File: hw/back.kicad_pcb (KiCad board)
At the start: 2 copper layers, 110 x 55 mm, 77 parts, among them J1 IDC_02X13, J2 FC681495, J3 N42GK-04, Q1 BSC080N03MS, U1 OSRB38C9BA, U2 MCP1826S, U3 MCP1826S, U4 BQ24192, U5 LTC1871, U6 LTC2941CMS8E

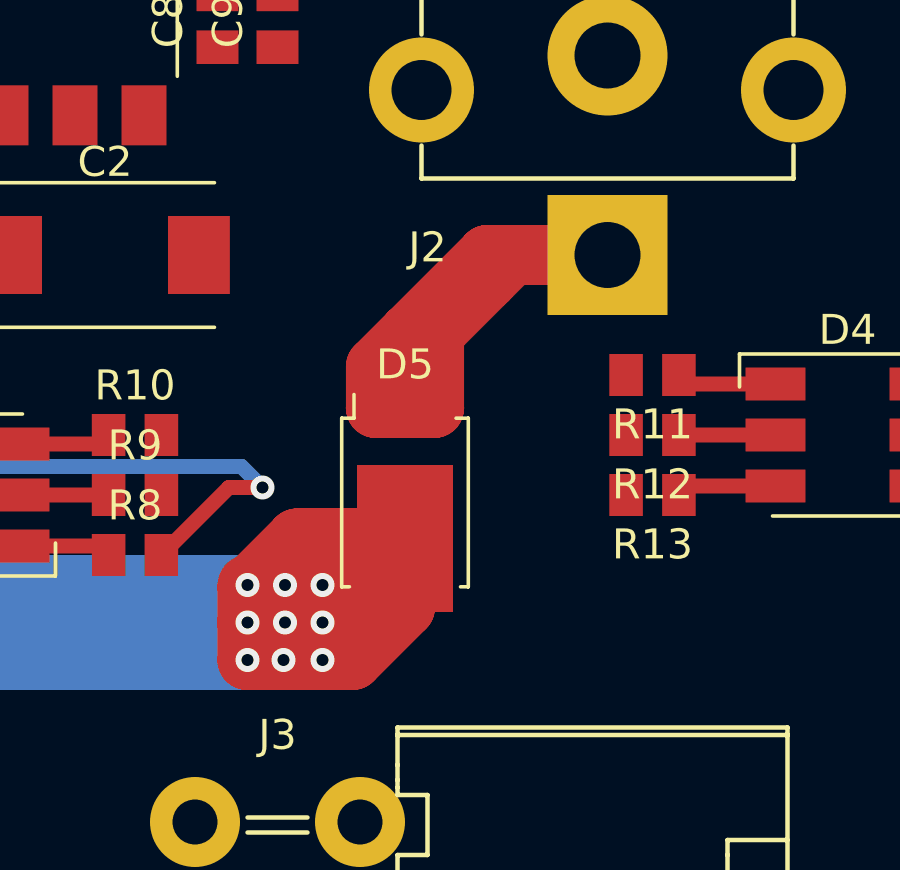
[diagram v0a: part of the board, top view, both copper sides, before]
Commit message: updated pcb
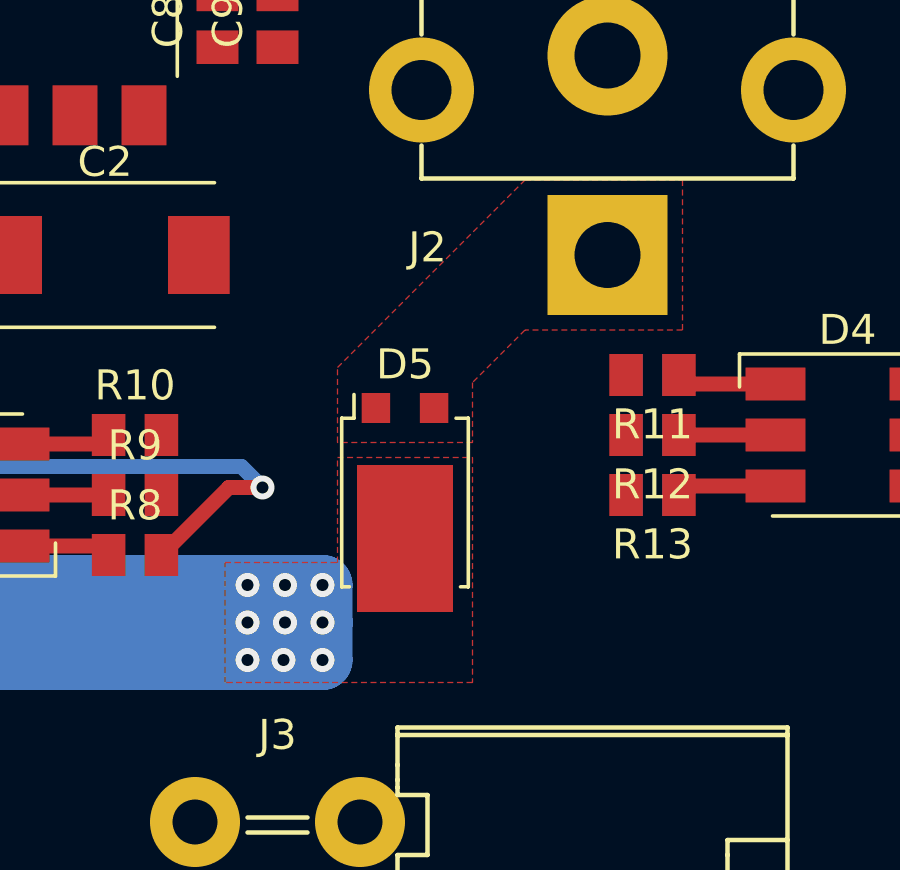
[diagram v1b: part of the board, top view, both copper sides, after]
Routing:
- net /charger/ADAPTER: track 191.2 -> 146.6 mm
- net Net-(D5-Pad1): track 25.3 -> 0.00 mm
- added copper zone on F.Cu, net /charger/ADAPTER
- added copper zone on F.Cu, net Net-(D5-Pad1)
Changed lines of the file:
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@@
     (thickness 1.6)
     (drawings 6)
-    (tracks 478)
+    (tracks 443)
     (zones 0)
     (modules 77)
@@
     (mod_text_size 1 1)
     (mod_text_width 0.15)
-    (pad_size 0.85 0.3)
-    (pad_drill 0)
+    (pad_size 4 4)
+    (pad_drill 2.2)
     (pad_to_mask_clearance 0.2)
     (aux_axis_origin 0 0)
@@
       (net 5 GND))
     (pad 1 thru_hole rect (at 0 -10.25 180) (size 4 4) (drill 2.2) (layers *.Cu *.Mask)
-      (net 8 "Net-(D5-Pad1)"))
+      (net 8 "Net-(D5-Pad1)") (zone_connect 2))
     (pad 2 thru_hole circle (at 0 -3.6 180) (size 4 4) (drill 2.2) (layers *.Cu *.Mask)
       (net 5 GND))
@@
       (net 8 "Net-(D5-Pad1)"))
     (pad 3 smd rect (at 0 1.2) (size 3.2 4.9) (layers F.Cu F.Mask)
-      (net 24 /charger/ADAPTER))
+      (net 24 /charger/ADAPTER) (zone_connect 2))
     (pad 1 smd rect (at -0.97 -3.15) (size 0.95 1) (layers F.Cu F.Paste F.Mask)
       (net 8 "Net-(D5-Pad1)"))
@@
   (segment (start 171.2 112.5) (end 172.5 112.5) (width 2) (layer B.Cu) (net 24))
   (segment (start 170 112.5) (end 171.2 112.5) (width 2) (layer B.Cu) (net 24))
-  (segment (start 171.2 112.5) (end 172.5 112.5) (width 2) (layer F.Cu) (net 24))
-  (segment (start 171.25 111.25) (end 171.25 110) (width 2) (layer F.Cu) (net 24))
-  (segment (start 172.5 111.25) (end 171.25 111.25) (width 2) (layer F.Cu) (net 24))
-  (segment (start 171.25 110) (end 172.5 110) (width 2) (layer F.Cu) (net 24))
-  (segment (start 170 110) (end 171.25 110) (width 2) (layer F.Cu) (net 24))
   (via (at 172.5 110) (size 0.8) (drill 0.4) (layers F.Cu B.Cu) (net 24))
   (via (at 171.25 110) (size 0.8) (drill 0.4) (layers F.Cu B.Cu) (net 24))
@@
   (via (at 172.5 111.25) (size 0.8) (drill 0.4) (layers F.Cu B.Cu) (net 24))
   (via (at 171.25 111.25) (size 0.8) (drill 0.4) (layers F.Cu B.Cu) (net 24))
-  (segment (start 170 111.25) (end 170 111.3) (width 2) (layer F.Cu) (net 24))
-  (segment (start 170 111.3) (end 171.2 112.5) (width 2) (layer F.Cu) (net 24))
   (via (at 171.2 112.5) (size 0.8) (drill 0.4) (layers F.Cu B.Cu) (net 24))
   (via (at 170 111.25) (size 0.8) (drill 0.4) (layers F.Cu B.Cu) (net 24))
-  (segment (start 171.65 108.45) (end 175.25 108.45) (width 2) (layer F.Cu) (net 24))
-  (segment (start 175.25 110.75) (end 173.5 112.5) (width 2) (layer F.Cu) (net 24))
-  (segment (start 173.5 112.5) (end 171.2 112.5) (width 2) (layer F.Cu) (net 24))
-  (segment (start 175.25 108.45) (end 175.25 110.75) (width 2) (layer F.Cu) (net 24))
-  (segment (start 172.75 108.45) (end 175.25 108.45) (width 2) (layer F.Cu) (net 24))
-  (segment (start 170 112.5) (end 170 111.25) (width 2) (layer F.Cu) (net 24))
-  (segment (start 170 111.2) (end 172.75 108.45) (width 2) (layer F.Cu) (net 24))
-  (segment (start 171.65 108.45) (end 172.75 108.45) (width 2) (layer F.Cu) (net 24))
-  (segment (start 170 111.25) (end 170 110.1) (width 2) (layer F.Cu) (net 24))
-  (segment (start 170 111.25) (end 170 111.2) (width 2) (layer F.Cu) (net 24))
-  (segment (start 170 110.1) (end 171.65 108.45) (width 2) (layer F.Cu) (net 24))
-  (segment (start 170 112.5) (end 171.2 112.5) (width 2) (layer F.Cu) (net 24))
-  (segment (start 171.2 112.5) (end 175.25 108.45) (width 2) (layer F.Cu) (net 24))
-  (segment (start 175.25 109.25) (end 172 112.5) (width 2) (layer F.Cu) (net 24))
-  (segment (start 172 112.5) (end 170 112.5) (width 2) (layer F.Cu) (net 24))
   (via (at 170 112.5) (size 0.8) (drill 0.4) (layers F.Cu B.Cu) (net 24))
   (segment (start 175.25 108.45) (end 175.25 109.25) (width 2) (layer F.Cu) (net 24))
@@
   (segment (start 155.25 94.3) (end 155.2 94.35) (width 1) (layer F.Cu) (net 4))
   (segment (start 161.943309 94.35) (end 161.95 94.343309) (width 1) (layer F.Cu) (net 4))
-  (segment (start 182 99) (end 178.82 99) (width 2) (layer F.Cu) (net 8))
-  (segment (start 178.82 99) (end 178 99.82) (width 2) (layer F.Cu) (net 8))
-  (segment (start 174.28 104.1) (end 174.28 102.72) (width 2) (layer F.Cu) (net 8))
-  (segment (start 174.28 102.72) (end 175.4 101.6) (width 2) (layer F.Cu) (net 8))
-  (segment (start 176.22 104.1) (end 176.22 101.6) (width 2) (layer F.Cu) (net 8))
-  (segment (start 176.22 101.6) (end 178 99.82) (width 2) (layer F.Cu) (net 8))
-  (segment (start 178 99.82) (end 178 99) (width 2) (layer F.Cu) (net 8))
-  (segment (start 174.28 104.1) (end 175.2 104.1) (width 2) (layer F.Cu) (net 8))
-  (segment (start 175.2 104.1) (end 176.22 104.1) (width 2) (layer F.Cu) (net 8))
-  (segment (start 175.4 101.6) (end 175.4 103.9) (width 2) (layer F.Cu) (net 8))
-  (segment (start 175.4 103.9) (end 175.2 104.1) (width 2) (layer F.Cu) (net 8))
-  (segment (start 182 99) (end 178 99) (width 2) (layer F.Cu) (net 8))
-  (segment (start 178 99) (end 175.4 101.6) (width 2) (layer F.Cu) (net 8))
   (segment (start 187.6 103.3) (end 184.68 103.3) (width 0.5) (layer F.Cu) (net 9))
   (segment (start 184.68 103.3) (end 184.38 103) (width 0.5) (layer F.Cu) (net 9))
@@
       )
     )
+  )
+  (zone (net 24) (net_name /charger/ADAPTER) (layer F.Cu) (hatch edge 0.508)
+    (priority 1)
+    (connect_pads (clearance 0.508))
+    (min_thickness 0.254)
+    (fill yes (arc_segments 16) (thermal_gap 0.508) (thermal_bridge_width 0.508))
+    (polygon
+      (pts
+        (xy 169.25 109.25) (xy 173 109.25) (xy 173 105.75) (xy 177.5 105.75) (xy 177.5 113.25)
+        (xy 169.25 113.25)
+      )
+    )
+  )
+  (zone (net 8) (net_name "Net-(D5-Pad1)") (layer F.Cu) (hatch edge 0.508)
+    (priority 2)
+    (connect_pads (clearance 0.508))
+    (min_thickness 0.254)
+    (fill yes (arc_segments 16) (thermal_gap 0.508) (thermal_bridge_width 0.508))
+    (polygon
+      (pts
+        (xy 173 102.75) (xy 179.25 96.5) (xy 184.5 96.5) (xy 184.5 101.5) (xy 179.25 101.5)
+        (xy 177.5 103.25) (xy 177.5 105.25) (xy 173 105.25)
+      )
+    )

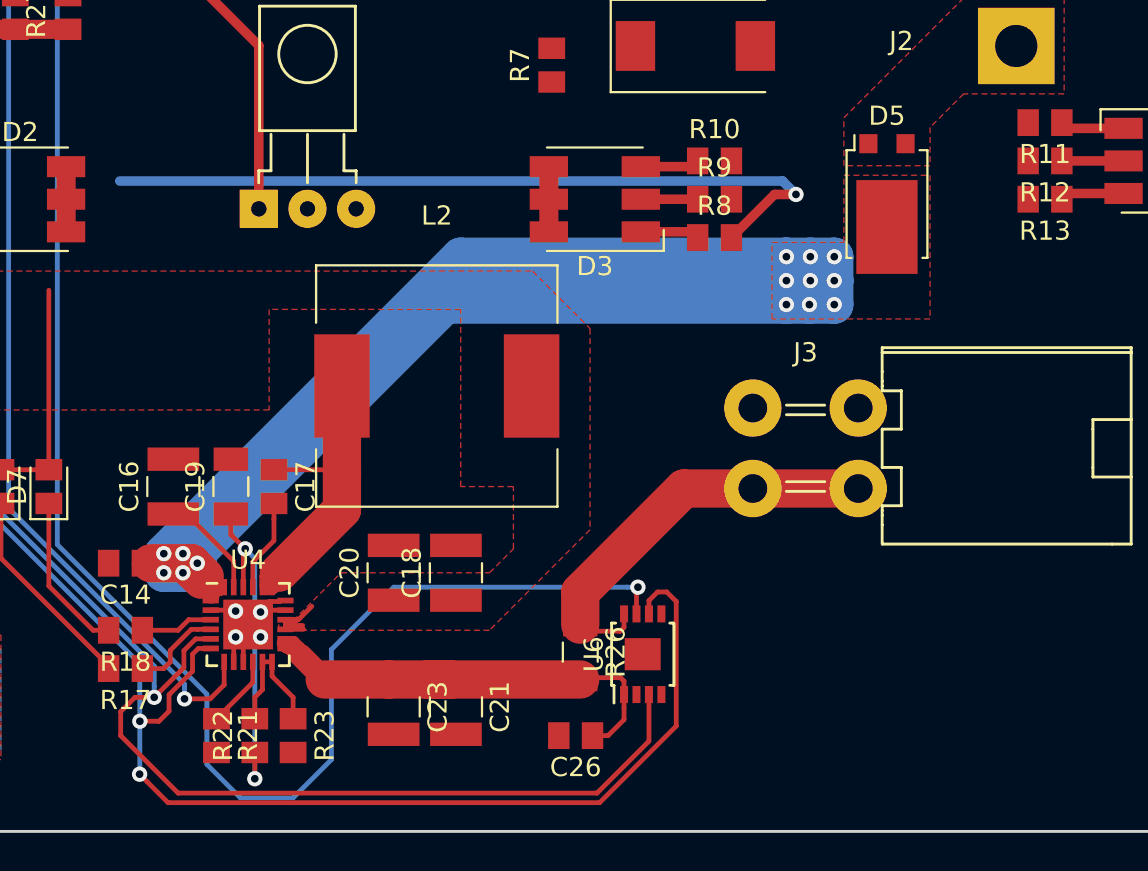
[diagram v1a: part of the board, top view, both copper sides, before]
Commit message: updated pcb
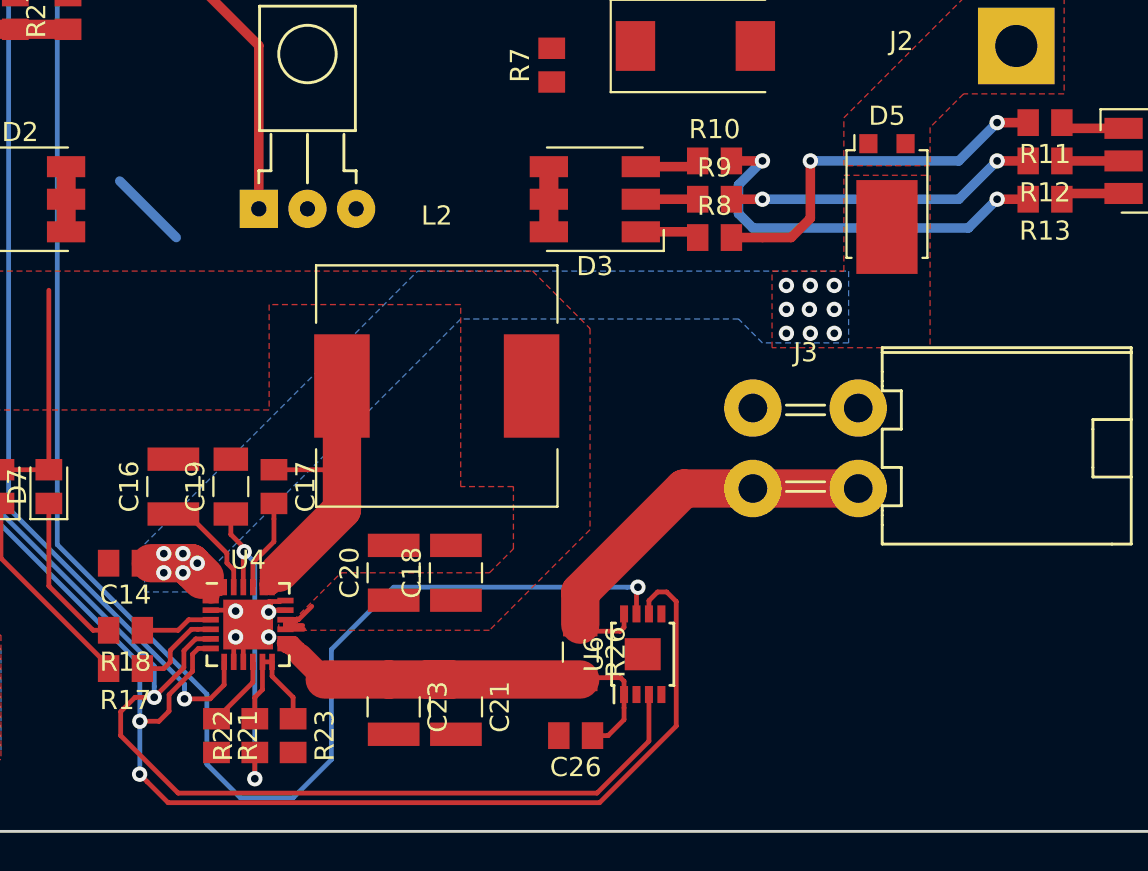
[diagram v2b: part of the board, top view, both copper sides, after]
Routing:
- net /charger/ADAPTER: track 146.6 -> 15.4 mm
- net /PWM_R: track 32.0 -> 52.9 mm, vias 0 -> 2
- net /PWM_G: track 42.5 -> 58.8 mm, vias 1 -> 3
- net /PWM_B: track 86.4 -> 70.4 mm, vias 2 -> 3
- added copper zone on B.Cu, net /charger/ADAPTER
